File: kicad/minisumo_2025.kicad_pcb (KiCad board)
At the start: 4 copper layers, 62.4 x 98 mm, 139 parts, among them J1 USB_C Connector, J10 DISTANCE_R90, J11 DISTANCE_R, J12 DISTANCE_RF, J13 DISTANCE_L90, J14 DISTANCE_L, J15 LINE_LEFT, J16 DISTANCE_LF, J3 START_MODULE, J4 MOTOR1, J5 MOTOR2, J6 BATT_IN, J8 DISTANCE_CENTER, J9 LINE_RIGHT, Q1 Si2371EDS, SW1 RESET, SW2 CASE, SW3 BOOT, U1 LMR33630ADDAR, U2 USBLC6-2P6, U3 ESP32-S3-WROOM-1, U4 TLV75733PDBVR, U5 TXS0108EPWR, U6 MC33926PNB, U7 MC33926PNB

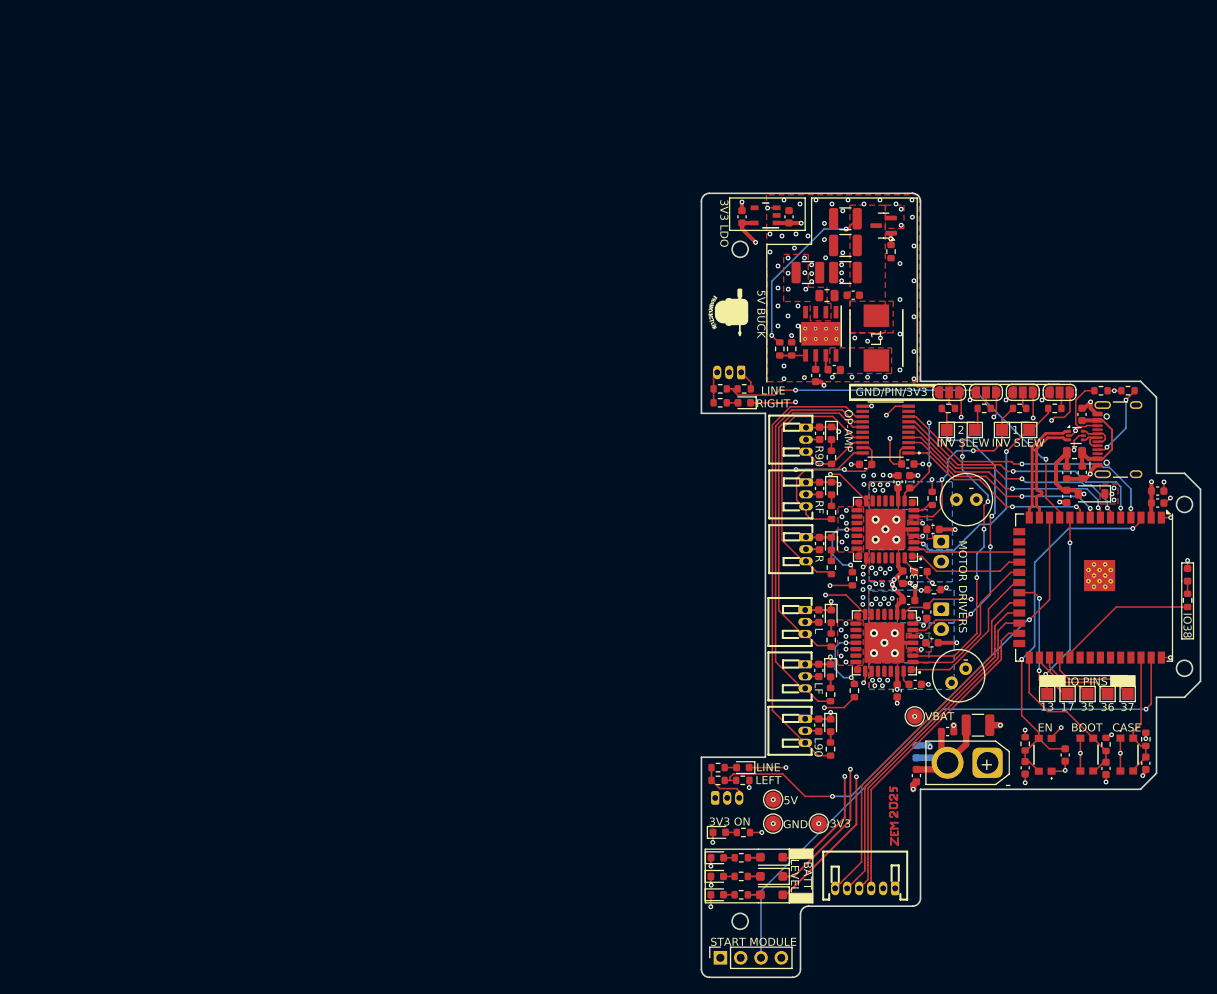
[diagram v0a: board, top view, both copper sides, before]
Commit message: 2026 version
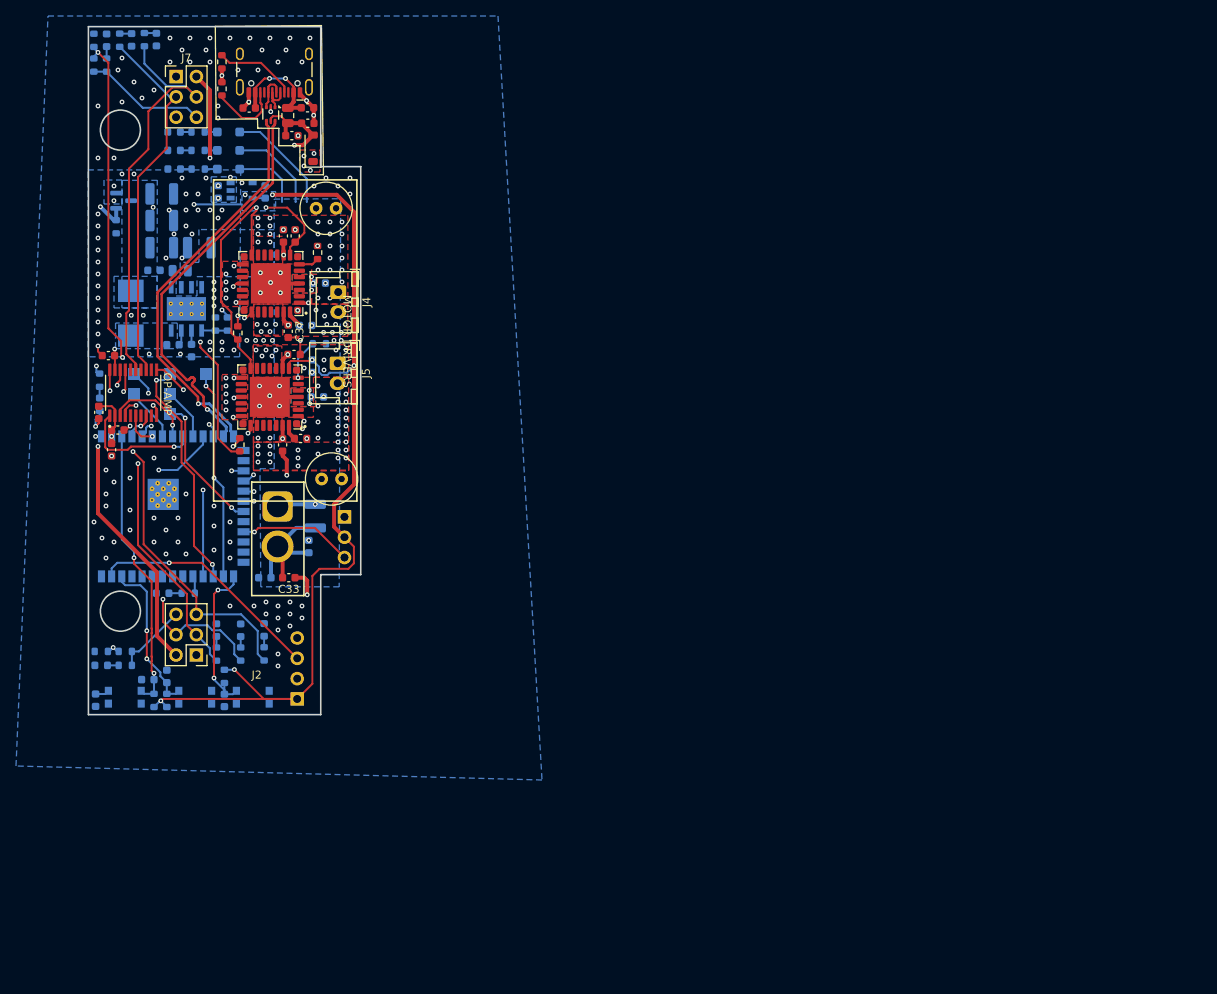
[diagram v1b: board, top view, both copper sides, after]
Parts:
- removed C44, C45, C46, C47, C48, C49: 0.1uF, Capacitor_SMD:C_0603_1608Metric
- removed D16: LED_Small, LED_SMD:LED_0603_1608Metric
- removed G***: LOGO, logos:logo
- removed J10: DISTANCE_R90, footprints:CONN-TH_S3B-ZR-3.4-LF-SN
- removed J11: DISTANCE_R, footprints:CONN-TH_S3B-ZR-3.4-LF-SN
- removed J12: DISTANCE_RF, footprints:CONN-TH_S3B-ZR-3.4-LF-SN
- removed J13: DISTANCE_L90, footprints:CONN-TH_S3B-ZR-3.4-LF-SN
- removed J14: DISTANCE_L, footprints:CONN-TH_S3B-ZR-3.4-LF-SN
- removed J15: LINE_LEFT, footprints:CONN-TH_S3B-ZR-3.4-LF-SN
- removed J16: DISTANCE_LF, footprints:CONN-TH_S3B-ZR-3.4-LF-SN
- removed J9: LINE_RIGHT, footprints:CONN-TH_S3B-ZR-3.4-LF-SN
- removed JP1, JP2, JP3, JP4: SolderJumper_3_Open, Jumper:SolderJumper-3_P1.3mm_Open_RoundedPad1.0x1.5mm_NumberLabels
- removed R10, R11, R12, R9: 1k, Resistor_SMD:R_0603_1608Metric
- removed R30: 3k3, Resistor_SMD:R_0603_1608Metric
- removed REF** (x4): TestPoint_Pad_D2.0mm, TestPoint:TestPoint_Pad_D2.0mm
- removed TP10: SLEW_2, TestPoint:TestPoint_Pad_1.5x1.5mm
- removed TP6: SLEW_1, TestPoint:TestPoint_Pad_1.5x1.5mm
- removed TP7: INV_1, TestPoint:TestPoint_Pad_1.5x1.5mm
- added J2: Conn_01x06_Pin, Connector_PinHeader_2.54mm:PinHeader_2x03_P2.54mm_Vertical, F.Cu at (44.3, 102.1)
- added J7: Conn_01x06_Pin, Connector_PinHeader_2.54mm:PinHeader_2x03_P2.54mm_Vertical, F.Cu at (41.8, 29.8)
- C10, C11, C12, C13, C14, C15, C18, C19, C23, C25, C27, C3, C31, C32, C35, C36, C4, C5, C7, C8, C9, D10, D11, D12, D13, D14, D15, D17, D18, D2, D4, D5, D6, D7, D8, D9, J3, J6, L1, Q1, R1, R16, R17, R18, R19, R20, R21, R22, R23, R24, R25, R26, R27, R28, R29, R31, R32, R33, R4, R5, R6, R7, R8, SW1, SW2, SW3, TP1, TP12, TP13, TP8, TP9, U1, U3, U4: moved to B.Cu
- C33, J4, J5: moved to F.Cu
- J8: value DISTANCE_CENTER -> Conn_01x03_Pin; footprint footprints:CONN-TH_S6B-ZR-3.4-LF-SN -> Connector_PinHeader_2.54mm:PinHeader_1x03_P2.54mm_Vertical; moved to B.Cu
- TP11: value INV_2 -> GPIO7; moved to B.Cu
- moved C2 130.9 mm to (33.7, 76.5), turned to -90 degrees
- moved TP12 130.5 mm to (36.5, 67.0), turned to 180 degrees
- moved C1 130.3 mm to (34.5, 74.0)
- moved D10 128.1 mm to (40.1, 94.4), turned to 0 degrees
- moved R28 125.5 mm to (34.7, 25.3)
- moved R19 124.9 mm to (43.3, 94.4), turned to 180 degrees
- moved TP9 123.8 mm to (41.0, 67.0), turned to 180 degrees
- moved R24 123.0 mm to (31.5, 25.3), turned to -90 degrees
- moved C18 122.9 mm to (40.6, 104.8), turned to 90 degrees
- moved R8 122.5 mm to (40.6, 107.8), turned to 90 degrees
- moved D14 122.4 mm to (36.2, 25.2), turned to 90 degrees
- moved C7 121.4 mm to (31.7, 107.8)
- moved D18 120.8 mm to (33.1, 25.3), turned to -90 degrees
- moved R2 120.5 mm to (47.5, 28.0), turned to 90 degrees
- moved R23 118.7 mm to (31.5, 28.4), turned to -90 degrees
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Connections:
- net /SENSORS/DISTANCE_RF_OUT renamed /SENSORS/DISTANCE_CENTER_OUT
- net DISTANCE_RF renamed DISTANCE_CENTER
- J8 pad 1: +3V3 -> GND
- J8 pad 2: GND -> +3V3
- J8 pad 3: GPIO48 -> GPIO21
- TP11 pad 1: /DRIVERS/INV_2 -> GPIO7
- U2 pad 1: D+ -> /POWER/D_N
- U2 pad 3: D- -> /POWER/D_P
- U2 pad 4: /POWER/D_N -> D+
- U2 pad 6: /POWER/D_P -> D-
- U3 pad 22: DISTANCE_INTR -> GPIO14
- U3 pad 5: DISTANCE_LF -> DISTANCE_R
- U3 pad 7: DISTANCE_R -> GPIO7
- U5 pad 14: /SENSORS/DISTANCE_LF_OUT -> unconnected-(U5-B6-Pad14)
- U5 pad 7: DISTANCE_LF -> unconnected-(U5-A6-Pad7)
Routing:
- net +3V3: track 79.2 -> 298.3 mm, vias 20 -> 13
- net +5V: track 27.6 -> 95.4 mm, vias 10 -> 11
- net GND: track 119.3 -> 57.8 mm, vias 143 -> 174
- net /SENSORS/DISTANCE_LF_OUT: track 50.7 -> 0.00 mm
- net DISTANCE_INTR: track 45.9 -> 0.00 mm
- net GPIO1: track 72.6 -> 29.4 mm
- net GPIO47: track 42.4 -> 0.00 mm
- net GPIO48: track 40.3 -> 0.00 mm
- net /DRIVERS/SLEW_2: track 39.3 -> 0.00 mm, vias 4 -> 0
- net /DRIVERS/INV_2: track 38.5 -> 0.00 mm, vias 4 -> 0
- net D+: track 14.4 -> 50.1 mm, vias 0 -> 1
- net D-: track 14.4 -> 50.0 mm, vias 0 -> 1
- net DISTANCE_LF: track 33.7 -> 0.00 mm, vias 2 -> 0
- net /SENSORS/DISTANCE_R90_OUT: track 8.82 -> 41.6 mm, vias 0 -> 2
- net DISTANCE_L90: track 35.1 -> 3.68 mm, vias 2 -> 1
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- added copper zone on B.Cu, net +3V3
- added copper zone on B.Cu, net +5V
- added copper zone on B.Cu, net +BATT
- added copper zone on In2.Cu, net /DRIVERS/MOTOR1_A
- added copper zone on In2.Cu, net /DRIVERS/MOTOR1_B
- added copper zone on In2.Cu, net /DRIVERS/MOTOR2_A
- added copper zone on In2.Cu, net /DRIVERS/MOTOR2_B
- added copper zone on B.Cu, net GND
- added copper zone on B.Cu, net Net-(Q1-D)
- added copper zone on B.Cu, net Net-(U1-SW)
- removed copper zone on In2.Cu, net +BATT
- removed copper zone on B.Cu, net /DRIVERS/MOTOR1_A
- removed copper zone on B.Cu, net /DRIVERS/MOTOR1_B
- removed copper zone on B.Cu, net /DRIVERS/MOTOR2_A
- removed copper zone on B.Cu, net /DRIVERS/MOTOR2_B
- removed copper zone on F.Cu, net Net-(Q1-D)
- removed copper zone on F.Cu, net Net-(U1-SW)
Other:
- board size 62.4 x 98 mm -> 34 x 86 mm
- board text added: "7"
- board text added: "C"
- board text added: "CASE LED"
- board text added: "SERVO"
- board text removed: "-"
- board text removed: "1"
- board text removed: "2"
- board text removed: "3V3"
- board text removed: "5V"
- board text removed: "GND"
- board text removed: "GND/PIN/3V3"
- board text removed: "INV"
- board text removed: "IO PINS"
- board text removed: "IO38"
- board text removed: "LF"
- board text removed: "RF"
- board text removed: "SLEW"
